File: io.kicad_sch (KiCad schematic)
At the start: 20 parts, among them J3 USB_C_Receptacle_USB2.0, J4 Conn_01x06_Male, U3 USBLC6-2SC6

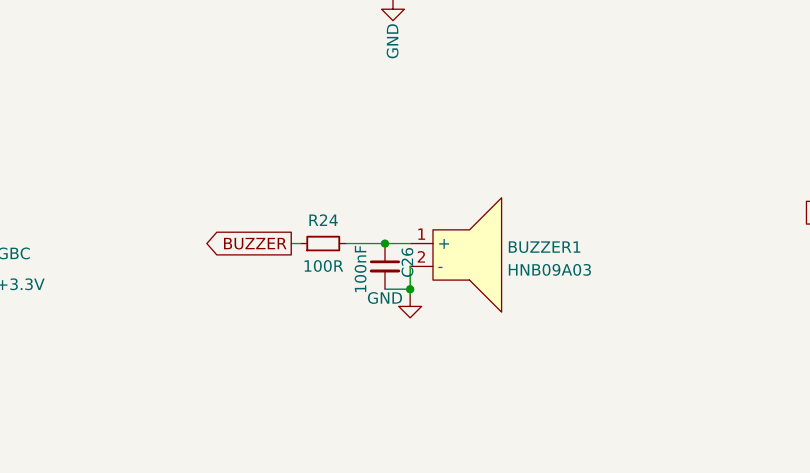
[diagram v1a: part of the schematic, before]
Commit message: Pcb with cutouts (#4)
* cut outs design in place

* kicad 8

* updated footprints

* publish v8

* image
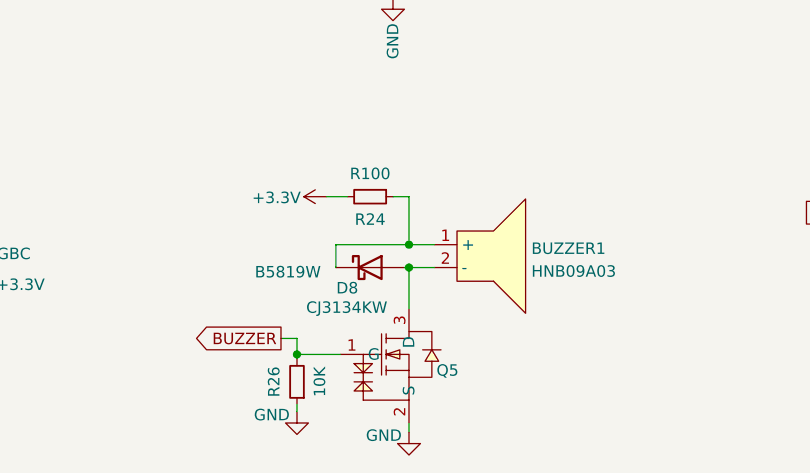
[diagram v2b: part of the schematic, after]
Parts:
- removed C26: 100nF, Capacitor_SMD:C_0402_1005Metric, symbol Device:C_Small
- added D8: B5819W, Diode_SMD:D_SOD-123, symbol Diode:MBR0530
- added Q5: CJ3134KW, easyeda2kicad:SC-70-3_L2.1-W1.3-P1.30-LS2.1-BR, symbol easyeda:CJ3134KW
- added R26: 10K, Resistor_SMD:R_0402_1005Metric, symbol Device:R_Small
- R24: value 100R -> R100; LCSC Part C106232 -> C191123
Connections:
- net +3.3V: now also R24.2
- net BUZZER: now also Q5.1 (G), R26.2; no longer R24.1
- net GND: now also Q5.2 (S), R26.1; no longer BUZZER1.2 (-)
- net at BUZZER1.1 (+): now also R24.1, D8.1 (K); no longer R24.2
- new net: BUZZER1.2 (-), D8.2 (A), Q5.3 (D)
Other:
- moved on the sheet: BUZZER1
